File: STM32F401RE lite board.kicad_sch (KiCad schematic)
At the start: 25 parts, among them J1 USB_B_Micro, J2 Conn_01x04_Pin, SW1 SW_Push, SW2 SW_SPDT, Y1 8MHz(16pF)

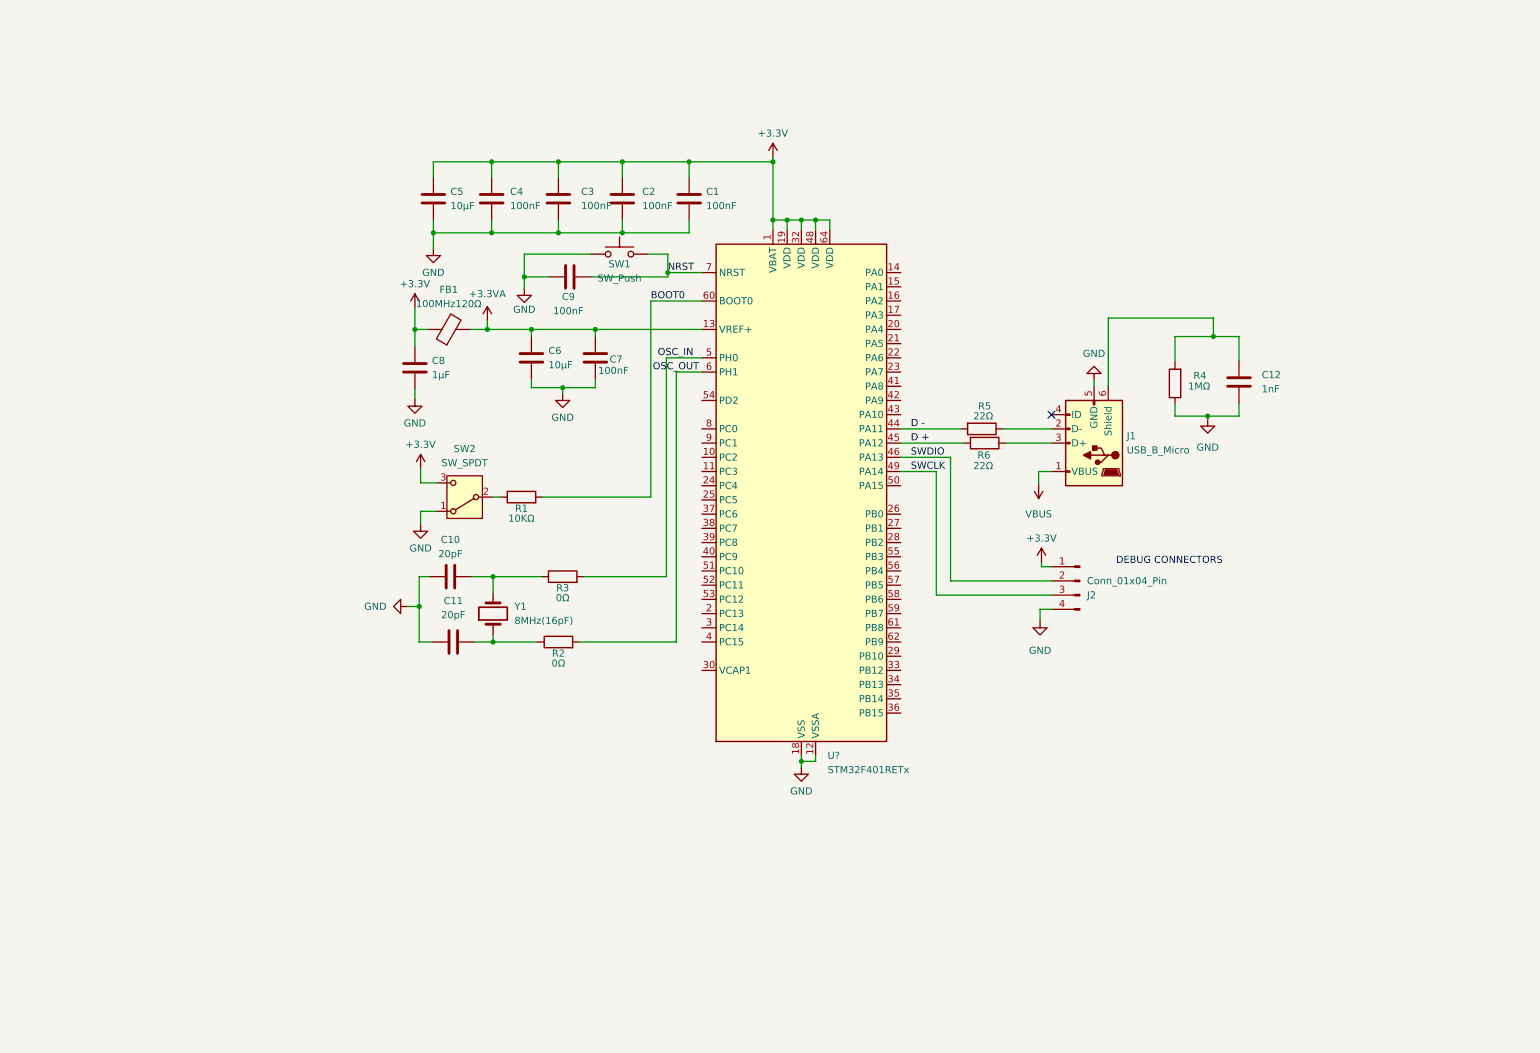
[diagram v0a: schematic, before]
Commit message: C1
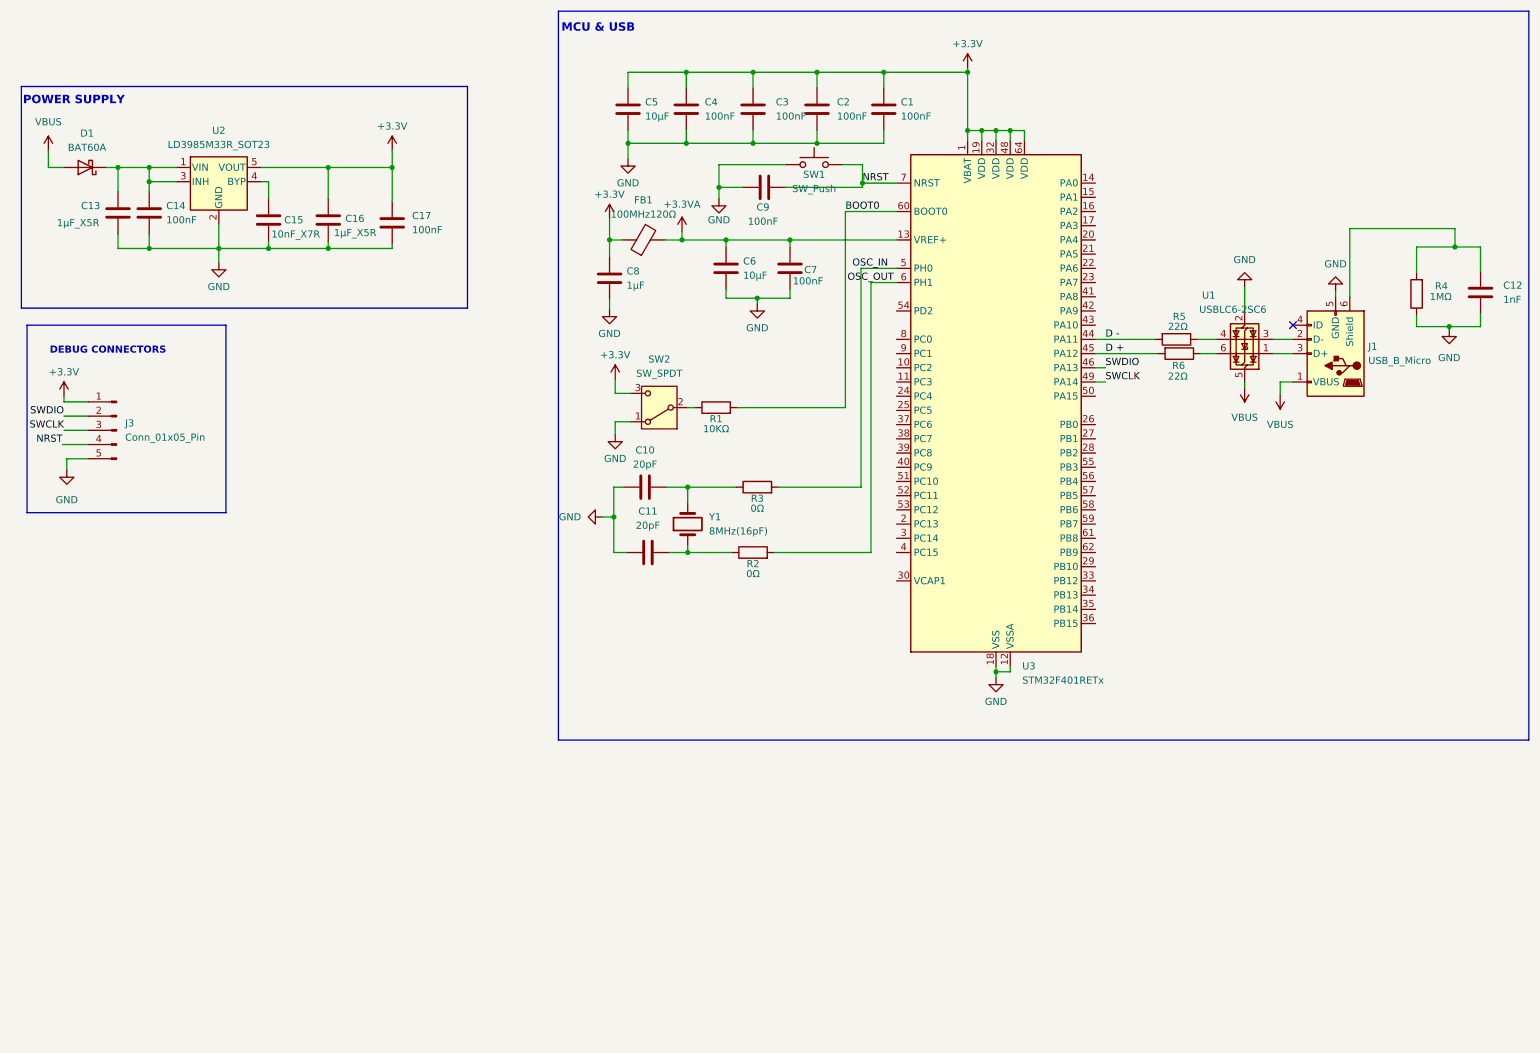
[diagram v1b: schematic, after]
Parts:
- removed J2: Conn_01x04_Pin, symbol Connector:Conn_01x04_Pin
- added C13, C16: 1µF_X5R, symbol Device:C
- added C14, C17: 100nF, symbol Device:C
- added C15: 10nF_X7R, symbol Device:C
- added D1: BAT60A, Diode_SMD:D_SOD-323, symbol Diode:BAT60A
- added J3: Conn_01x05_Pin, symbol Connector:Conn_01x05_Pin
- added U1: USBLC6-2SC6, Package_TO_SOT_SMD:SOT-23-6, symbol Power_Protection:USBLC6-2SC6
- added U2: LD3985M33R_SOT23, Package_TO_SOT_SMD:SOT-23-5, symbol Regulator_Linear:LD3985M33R_SOT23
- gave numbers to parts that had none: 1
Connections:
- net +3.3V: now also C16.1, C17.1, J3.1 (Pin_1), U2.5 (VOUT)
- net GND: now also C13.2, C14.2, C15.2, C16.2, C17.2, J3.5 (Pin_5), U1.2 (GND), U2.2 (GND)
- net NRST: now also J3.4 (Pin_4)
- net SWCLK: now also J3.3 (Pin_3)
- net SWDIO: now also J3.2 (Pin_2)
- net VBUS: now also D1.2 (A), U1.5 (VBUS)
- net at R6.1: now also U1.6 (I/O1); no longer J1.3 (D+)
- net at J1.2 (D-): now also U1.3 (I/O2); no longer R5.1
- new net: C13.1, C14.1, D1.1 (K), U2.1 (VIN), U2.3 (INH)
- new net: C15.1, U2.4 (BYP)
- new net: J1.3 (D+), U1.1 (I/O1)
- new net: R5.1, U1.4 (I/O2)
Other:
- note added: "MCU & USB"
- note added: "POWER SUPPLY"
- moved on the sheet: C1, C10, C11, C12, C2, C3, C4, C5, C6, C7, C8, C9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

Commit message: C2
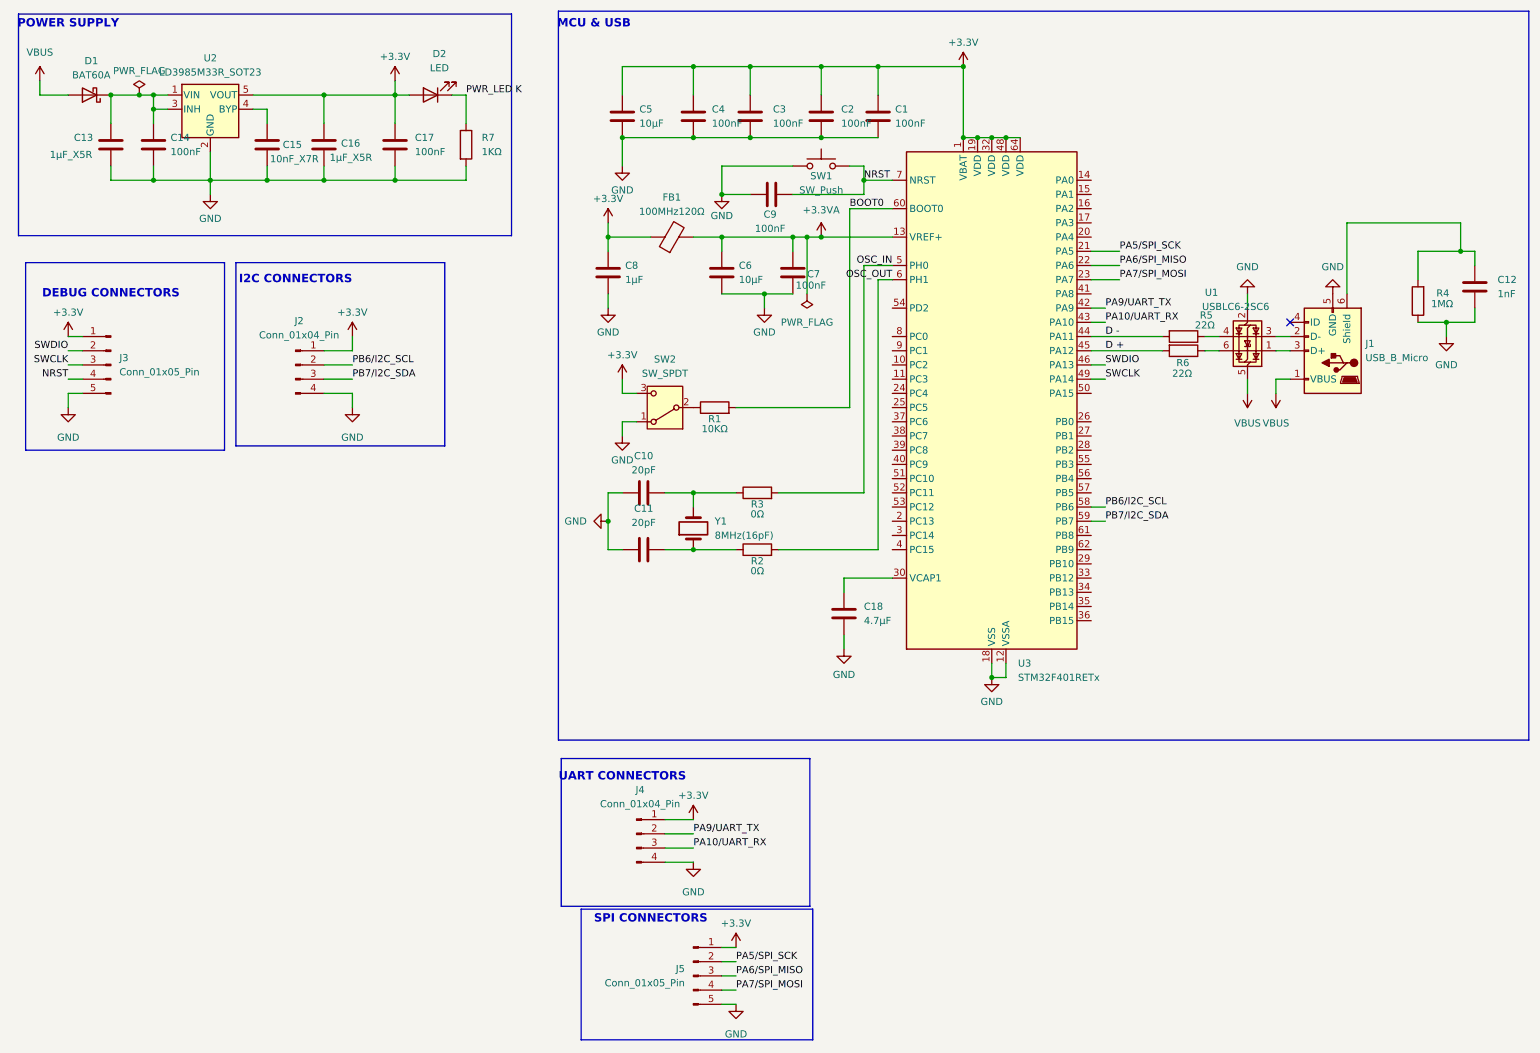
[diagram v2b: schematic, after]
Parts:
- added C18: 4.7µF, symbol Device:C
- added D2: LED, symbol Device:LED
- added J2, J4: Conn_01x04_Pin, symbol Connector:Conn_01x04_Pin
- added J5: Conn_01x05_Pin, symbol Connector:Conn_01x05_Pin
- added R7: 1KΩ, symbol Device:R
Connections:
- net +3.3V: now also D2.2 (A), J2.1 (Pin_1), J4.1 (Pin_1), J5.1 (Pin_1)
- net GND: now also C18.2, J2.4 (Pin_4), J4.4 (Pin_4), J5.5 (Pin_5), R7.2
- net PA5/SPI_SCK: now reaches U3.21 (PA5)
- net PA5/SPI_SCK: now also J5.2 (Pin_2)
- net PA6/SPI_MISO: now reaches U3.22 (PA6)
- net PA6/SPI_MISO: now also J5.3 (Pin_3)
- net PA7/SPI_MOSI: now reaches U3.23 (PA7)
- net PA7/SPI_MOSI: now also J5.4 (Pin_4)
- net at U3.30 (VCAP1): now also C18.1
- net PA9/UART_TX: now reaches U3.42 (PA9)
- net PA9/UART_TX: now also J4.2 (Pin_2)
- net PA10/UART_RX: now reaches U3.43 (PA10)
- net PA10/UART_RX: now also J4.3 (Pin_3)
- net PB6/I2C_SCL: now reaches U3.58 (PB6)
- net PB6/I2C_SCL: now also J2.2 (Pin_2)
- net PB7/I2C_SDA: now reaches U3.59 (PB7)
- net PB7/I2C_SDA: now also J2.3 (Pin_3)
- new net PWR_LED K: D2.1 (K), R7.1
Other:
- note added: "I2C CONNECTORS"
- note added: "SPI CONNECTORS"
- note added: "UART CONNECTORS"
- moved on the sheet: C1, C10, C11, C12, C13, C14, C15, C16, C17, C2, C3, C4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
